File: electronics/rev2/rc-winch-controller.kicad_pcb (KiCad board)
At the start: 2 copper layers, 30 x 16 mm, 13 parts, among them J1 Conn_01x06, J2 Conn_01x06, SW1 SETUP, U1 ME6209A33M3G, U2 LPC812M101JDH20, U3 RZ7889

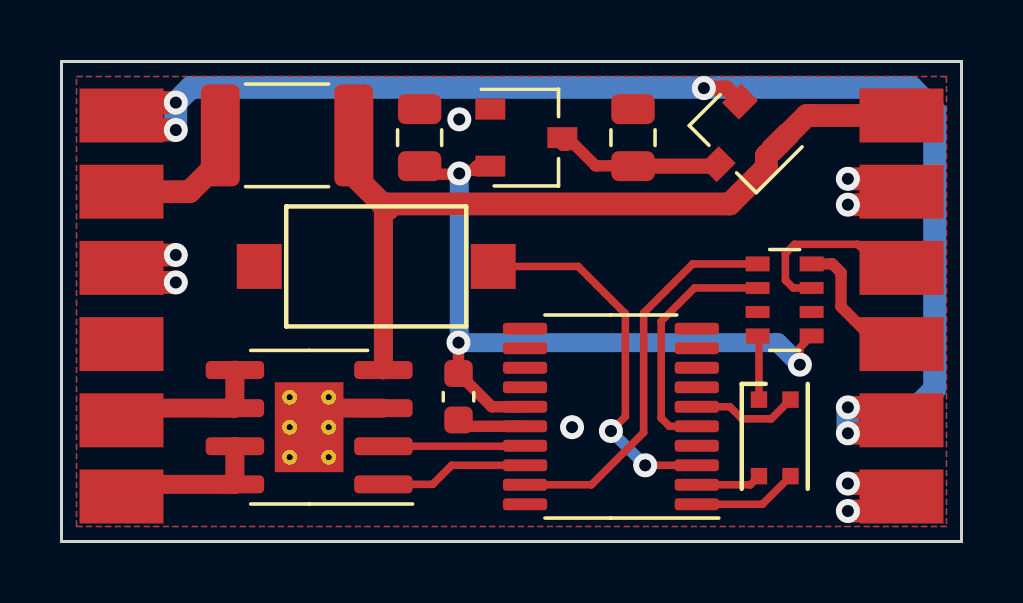
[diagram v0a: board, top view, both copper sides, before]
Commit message: Improve layout
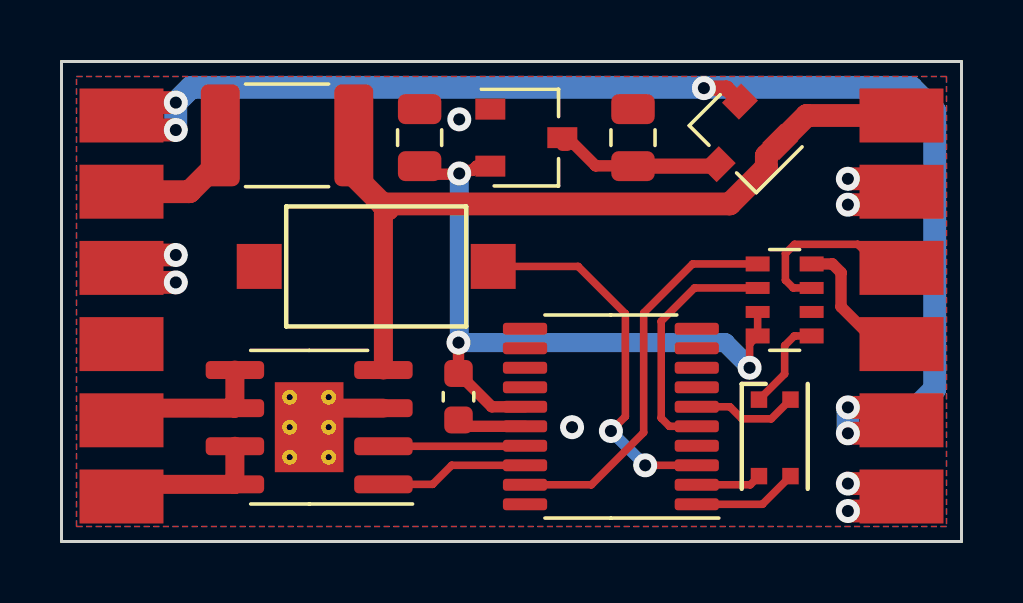
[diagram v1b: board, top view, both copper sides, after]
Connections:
- RN1 pad 1: +3V3 -> /LED-A
- RN1 pad 7: (no net) -> +3V3
- RN1 pad 8: /LED-A -> +3V3
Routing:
- net /LED-A: track 2.14 -> 3.19 mm
- net +3V3: track 24.8 -> 24.0 mm
